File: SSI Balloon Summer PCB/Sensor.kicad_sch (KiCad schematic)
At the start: 16 parts, among them J8 PT1000 Sensor, U10 MS5611-01BA03, U4 ICM-42688-P, U9 MAX31865ATP_T

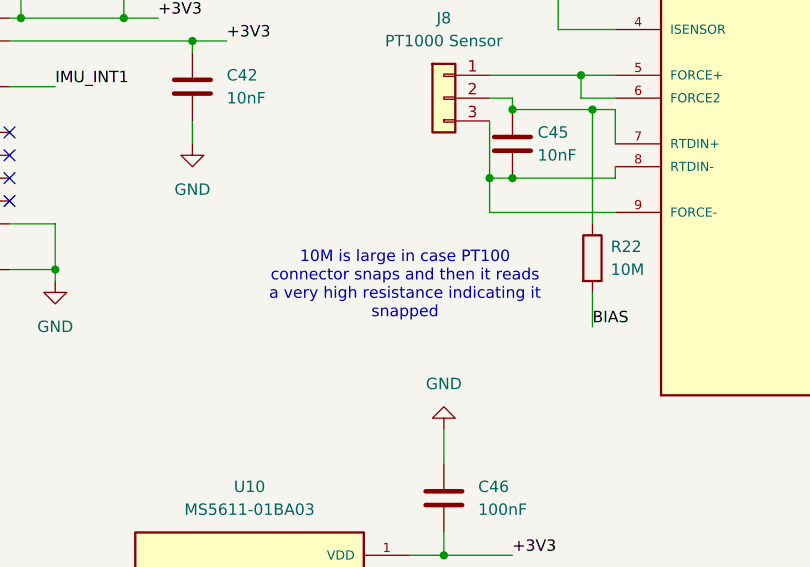
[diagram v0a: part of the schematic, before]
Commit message: Reviewed sensor sheet
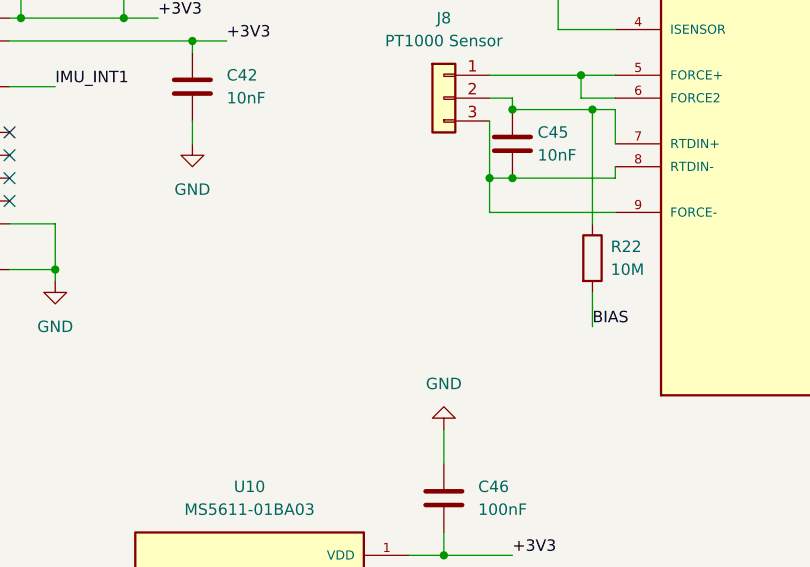
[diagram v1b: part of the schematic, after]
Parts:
- C11, C12, C42, C43, C44, C45, C46: footprint Capacitor_SMD:C_0603_1608Metric -> (none)
- J8: footprint Connector_JST:JST_PH_B3B-PH-K_1x03_P2.00mm_Vertical -> (none)
- R21, R22, R23, R24, R25: footprint Resistor_SMD:R_0603_1608Metric -> (none)
- U4: footprint ICM-42688-P 2:PQFN50P300X250X97-14N -> ICM-42688-P:PQFN50P300X250X97-14N
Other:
- note removed: "10M is large in case PT100 connector snaps and then it reads a very high resistance indicating it snapped"
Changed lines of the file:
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@@
 		)
 	)
-	(text "10M is large in case PT100\nconnector snaps and then it reads\na very high resistance indicating it\nsnapped"
-		(exclude_from_sim no)
-		(at 146.812 113.538 0)
-		(effects
-			(font
-				(size 1.27 1.27)
-			)
-		)
-	)
 	(text "Input:"
 		(exclude_from_sim no)
@@
 			)
 		)
-		(property "Footprint" "Resistor_SMD:R_0603_1608Metric"
+		(property "Footprint" ""
 			(at 220.218 97.79 90)
 			(hide yes)
@@
 			)
 		)
-		(property "Footprint" "Resistor_SMD:R_0603_1608Metric"
+		(property "Footprint" ""
 			(at 37.338 101.6 90)
 			(hide yes)
@@
 			)
 		)
-		(property "Footprint" "Resistor_SMD:R_0603_1608Metric"
+		(property "Footprint" ""
 			(at 153.67 79.248 90)
 			(hide yes)
@@
 			)
 		)
-		(property "Footprint" "Capacitor_SMD:C_0603_1608Metric"
+		(property "Footprint" ""
 			(at 116.5352 81.28 0)
 			(hide yes)
@@
 			)
 		)
-		(property "Footprint" "Capacitor_SMD:C_0603_1608Metric"
+		(property "Footprint" ""
 			(at 105.1052 81.28 0)
 			(hide yes)
@@
 			)
 		)
-		(property "Footprint" "ICM-42688-P 2:PQFN50P300X250X97-14N"
+		(property "Footprint" "ICM-42688-P:PQFN50P300X250X97-14N"
 			(at 77.47 96.52 0)
 			(hide yes)
@@
 			)
 		)
-		(property "Footprint" "Resistor_SMD:R_0603_1608Metric"
+		(property "Footprint" ""
 			(at 97.028 156.21 90)
 			(hide yes)
@@
 			)
 		)
-		(property "Footprint" "Resistor_SMD:R_0603_1608Metric"
+		(property "Footprint" ""
 			(at 165.862 110.49 90)
 			(hide yes)
@@
 			)
 		)
-		(property "Footprint" "Capacitor_SMD:C_0603_1608Metric"
+		(property "Footprint" ""
 			(at 152.0952 140.97 0)
 			(hide yes)
@@
 			)
 		)
-		(property "Footprint" "Capacitor_SMD:C_0603_1608Metric"
+		(property "Footprint" ""
 			(at 229.5652 68.58 0)
 			(hide yes)
@@
 			)
 		)
-		(property "Footprint" "Capacitor_SMD:C_0603_1608Metric"
+		(property "Footprint" ""
 			(at 159.7152 101.6 0)
 			(hide yes)
@@
 			)
 		)
-		(property "Footprint" "Capacitor_SMD:C_0603_1608Metric"
+		(property "Footprint" ""
 			(at 229.5652 81.28 0)
 			(hide yes)
@@
 			)
 		)
-		(property "Footprint" "Capacitor_SMD:C_0603_1608Metric"
+		(property "Footprint" ""
 			(at 124.1552 95.25 0)
 			(hide yes)
@@
 			)
 		)
-		(property "Footprint" "Connector_JST:JST_PH_B3B-PH-K_1x03_P2.00mm_Vertical"
+		(property "Footprint" ""
 			(at 151.13 92.71 0)
 			(hide yes)

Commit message: Layout placement for every sheet except PWR and SD card
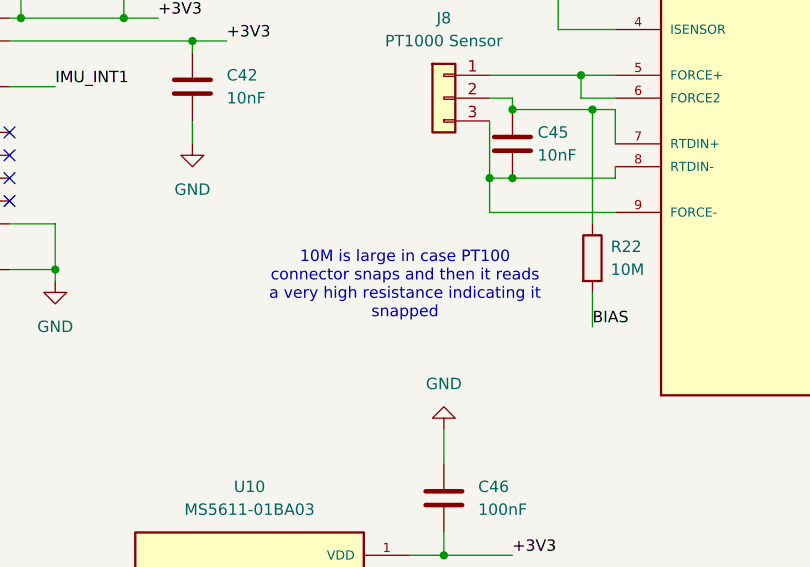
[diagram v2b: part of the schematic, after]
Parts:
- C11, C12, C42, C43, C44, C45, C46: footprint (none) -> Capacitor_SMD:C_0603_1608Metric
- J8: footprint (none) -> Connector_JST:JST_PH_B3B-PH-K_1x03_P2.00mm_Vertical
- R21, R22, R23, R24, R25: footprint (none) -> Resistor_SMD:R_0603_1608Metric
- U4: footprint ICM-42688-P:PQFN50P300X250X97-14N -> ICM-42688-P 2:PQFN50P300X250X97-14N
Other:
- note added: "10M is large in case PT100 connector snaps and then it reads a very high resistance indicating it snapped"
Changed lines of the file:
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@@
 		)
 	)
+	(text "10M is large in case PT100\nconnector snaps and then it reads\na very high resistance indicating it\nsnapped"
+		(exclude_from_sim no)
+		(at 146.812 113.538 0)
+		(effects
+			(font
+				(size 1.27 1.27)
+			)
+		)
+	)
 	(text "Input:"
 		(exclude_from_sim no)
@@
 			)
 		)
-		(property "Footprint" ""
+		(property "Footprint" "Resistor_SMD:R_0603_1608Metric"
 			(at 220.218 97.79 90)
 			(hide yes)
@@
 			)
 		)
-		(property "Footprint" ""
+		(property "Footprint" "Resistor_SMD:R_0603_1608Metric"
 			(at 37.338 101.6 90)
 			(hide yes)
@@
 			)
 		)
-		(property "Footprint" ""
+		(property "Footprint" "Resistor_SMD:R_0603_1608Metric"
 			(at 153.67 79.248 90)
 			(hide yes)
@@
 			)
 		)
-		(property "Footprint" ""
+		(property "Footprint" "Capacitor_SMD:C_0603_1608Metric"
 			(at 116.5352 81.28 0)
 			(hide yes)
@@
 			)
 		)
-		(property "Footprint" ""
+		(property "Footprint" "Capacitor_SMD:C_0603_1608Metric"
 			(at 105.1052 81.28 0)
 			(hide yes)
@@
 			)
 		)
-		(property "Footprint" "ICM-42688-P:PQFN50P300X250X97-14N"
+		(property "Footprint" "ICM-42688-P 2:PQFN50P300X250X97-14N"
 			(at 77.47 96.52 0)
 			(hide yes)
@@
 			)
 		)
-		(property "Footprint" ""
+		(property "Footprint" "Resistor_SMD:R_0603_1608Metric"
 			(at 97.028 156.21 90)
 			(hide yes)
@@
 			)
 		)
-		(property "Footprint" ""
+		(property "Footprint" "Resistor_SMD:R_0603_1608Metric"
 			(at 165.862 110.49 90)
 			(hide yes)
@@
 			)
 		)
-		(property "Footprint" ""
+		(property "Footprint" "Capacitor_SMD:C_0603_1608Metric"
 			(at 152.0952 140.97 0)
 			(hide yes)
@@
 			)
 		)
-		(property "Footprint" ""
+		(property "Footprint" "Capacitor_SMD:C_0603_1608Metric"
 			(at 229.5652 68.58 0)
 			(hide yes)
@@
 			)
 		)
-		(property "Footprint" ""
+		(property "Footprint" "Capacitor_SMD:C_0603_1608Metric"
 			(at 159.7152 101.6 0)
 			(hide yes)
@@
 			)
 		)
-		(property "Footprint" ""
+		(property "Footprint" "Capacitor_SMD:C_0603_1608Metric"
 			(at 229.5652 81.28 0)
 			(hide yes)
@@
 			)
 		)
-		(property "Footprint" ""
+		(property "Footprint" "Capacitor_SMD:C_0603_1608Metric"
 			(at 124.1552 95.25 0)
 			(hide yes)
@@
 			)
 		)
-		(property "Footprint" ""
+		(property "Footprint" "Connector_JST:JST_PH_B3B-PH-K_1x03_P2.00mm_Vertical"
 			(at 151.13 92.71 0)
 			(hide yes)
